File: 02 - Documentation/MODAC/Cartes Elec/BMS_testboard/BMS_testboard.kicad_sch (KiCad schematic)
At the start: 33 parts, among them J1 2P Droit 22-11-2022, J2 6P Droit 22-11-2062, J3 6P Droit 22-11-2062, J4 2P Droit 22-11-2022, Q1 NMOS SQ2348ES-T1_GE3, Q10 PMOS SI2343CDS-T1-GE3, Q11 NMOS SQ2348ES-T1_GE3, Q12 PMOS SI2343CDS-T1-GE3, Q13 NMOS SQ2348ES-T1_GE3, Q14 NMOS SQ2348ES-T1_GE3, Q15 PMOS SI2343CDS-T1-GE3, Q16 PMOS SI2343CDS-T1-GE3, Q17 NMOS SQ2348ES-T1_GE3, Q18 NMOS SQ2348ES-T1_GE3, Q19 PMOS SI2343CDS-T1-GE3, Q2 PMOS SI2343CDS-T1-GE3, Q20 PMOS SI2343CDS-T1-GE3, Q21 NMOS SQ2348ES-T1_GE3, Q22 NMOS SQ2348ES-T1_GE3, Q23 PMOS SI2343CDS-T1-GE3, Q24 PMOS SI2343CDS-T1-GE3, Q3 NMOS SQ2348ES-T1_GE3, Q4 PMOS SI2343CDS-T1-GE3, Q5 NMOS SQ2348ES-T1_GE3, Q6 PMOS SI2343CDS-T1-GE3, Q7 NMOS SQ2348ES-T1_GE3, Q8 PMOS SI2343CDS-T1-GE3, Q9 NMOS SQ2348ES-T1_GE3, U1 ADG406BPZ

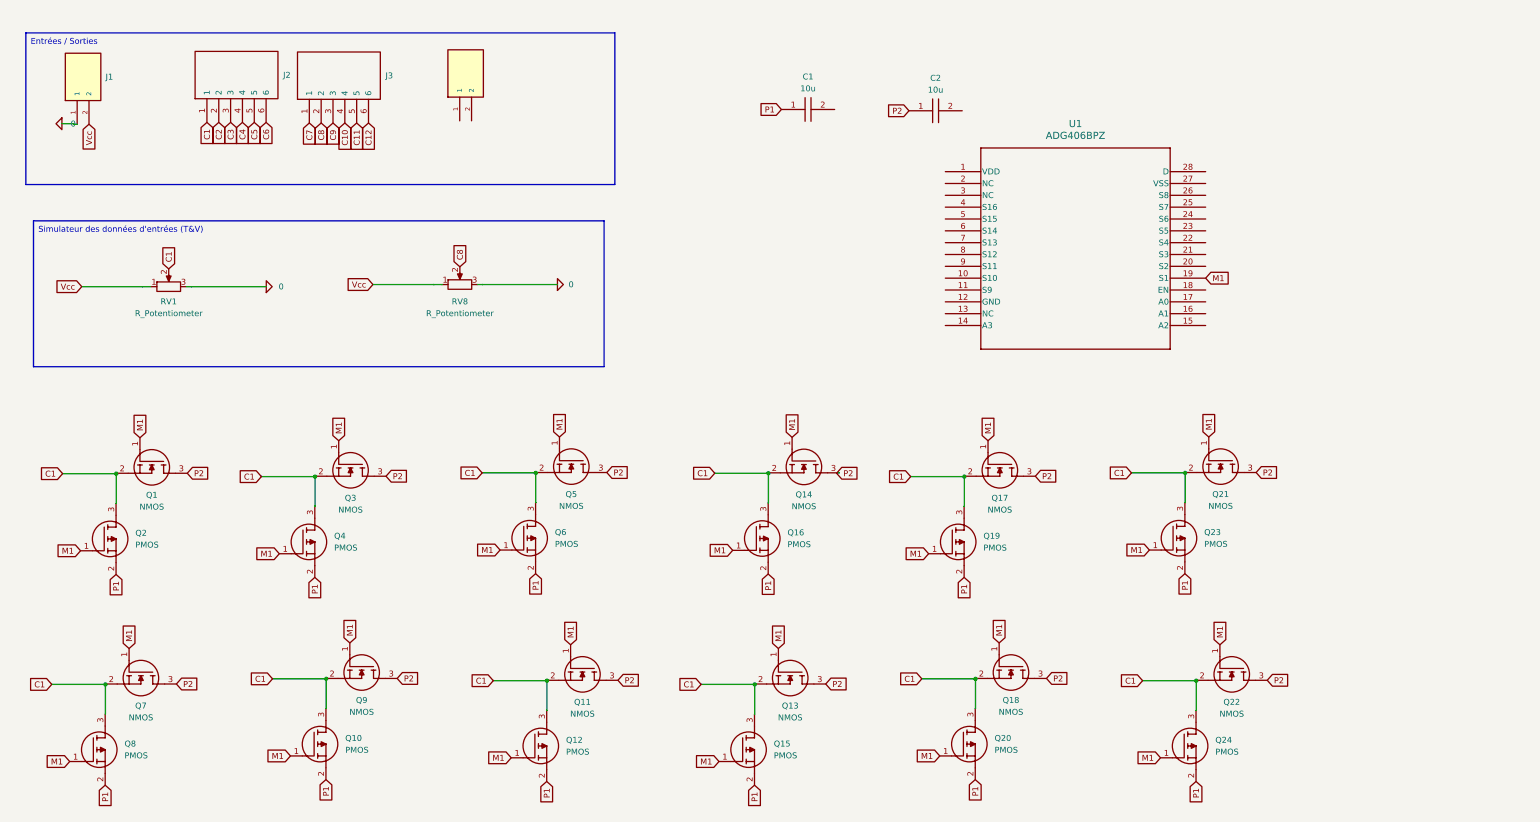
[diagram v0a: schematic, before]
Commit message: BOMs et BMS Testboard
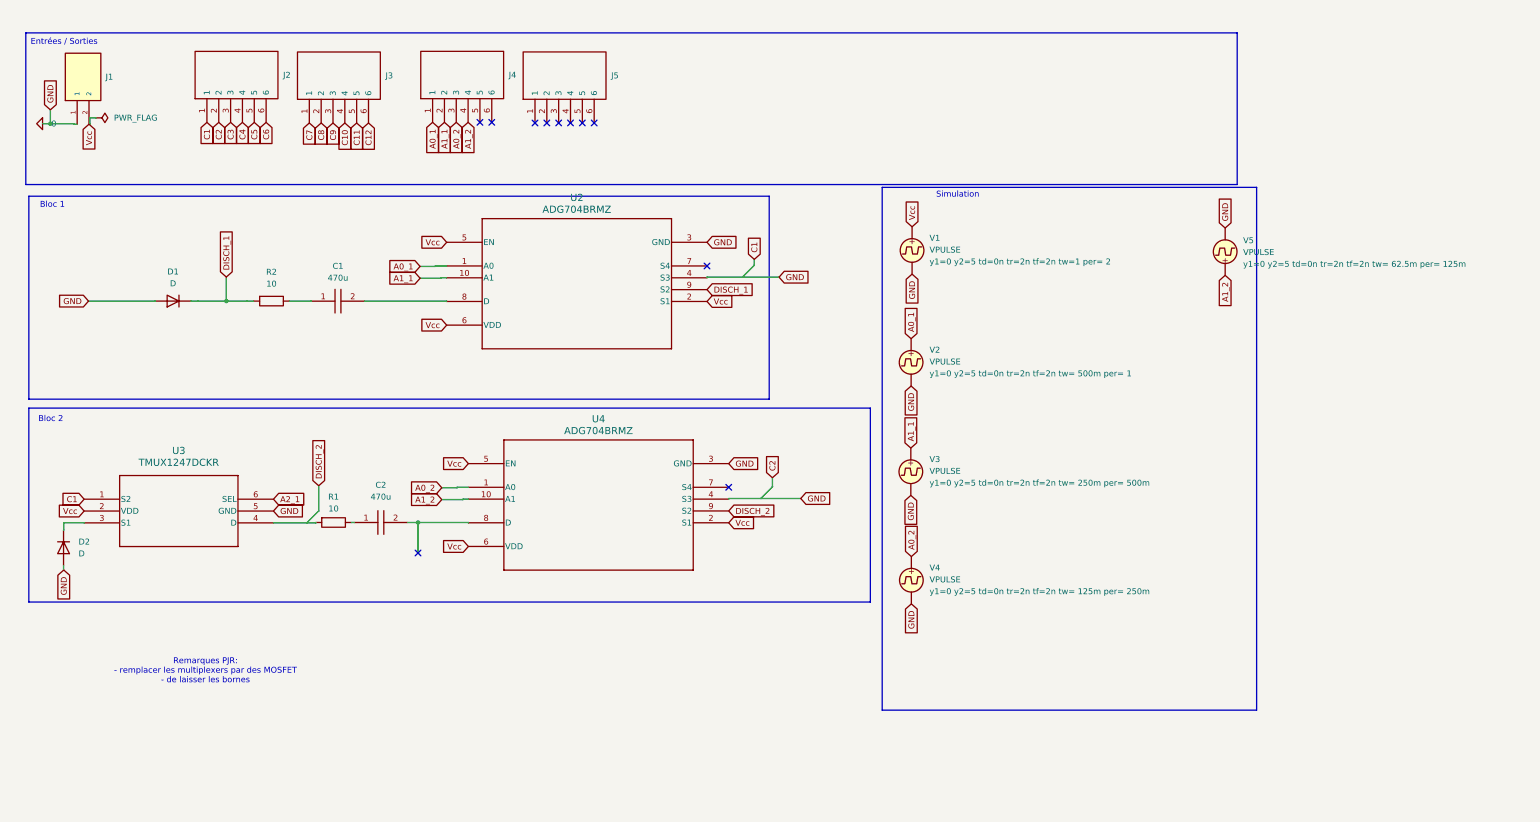
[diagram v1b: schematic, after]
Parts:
- removed J4: 2P Droit 22-11-2022, EPSA_lib:MOLEX_22-11-2022, symbol EPSA_lib:2P Droit 22-11-2022
- removed Q1, Q11, Q13, Q14, Q17, Q18, Q21, Q22, Q3, Q5, Q7, Q9: NMOS SQ2348ES-T1_GE3, EPSA_lib:SOT95P237X112-3N, symbol EPSA_lib:NMOS SQ2348ES-T1_GE3
- removed Q10, Q12, Q15, Q16, Q19, Q2, Q20, Q23, Q24, Q4, Q6, Q8: PMOS SI2343CDS-T1-GE3, EPSA_lib:SOT95P237X112-3N, symbol EPSA_lib:PMOS SI2343CDS-T1-GE3
- removed RV1, RV8: R_Potentiometer, symbol Device:R_Potentiometer
- removed U1: ADG406BPZ, P_28_ADI, symbol Multiplexer_16channels:ADG406BPZ
- added D1, D2: D, symbol Device:D
- added J4, J5: 6P Droit 22-11-2062, EPSA_lib:HDRV6W87P0X254_1X6_1509X635X1092P, symbol EPSA_lib:6P Droit 22-11-2062
- added R1, R2: 10, symbol Device:R
- added U2, U4: ADG704BRMZ, RM_10_ADI, symbol 2025-02-14_19-46-42:ADG704BRMZ
- added U3: TMUX1247DCKR, SOT-SC70_DCK_6_TEX, symbol 2025-02-14_19-49-50:TMUX1247DCKR
- added V1, V2, V3, V4, V5: VPULSE, symbol Simulation_SPICE:VPULSE
- C1, C2: value 10u -> 470u
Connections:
- net 0: now also D1.2 (A), D2.2 (A), U2.3 (GND), U2.4 (S3), U3.5 (GND), U4.3 (GND), U4.4 (S3), V1.2, V2.2, V3.2, V4.2, V5.2
- net C1: now also U3.1 (S2)
- net Vcc: now also U2.2 (S1), U2.5 (EN), U2.6 (VDD), U3.2 (VDD), U4.2 (S1), U4.5 (EN), U4.6 (VDD), V1.1
- net at C2.2: now also U4.8 (D)
- net at C1.2: now also U2.8 (D)
- net P1: no longer names the net of C1.1
- net P1: now also R2.1
- net P2: no longer names the net of C2.1
- net P2: now also R1.1
- new net: R1.2, U3.4 (D)
- new net: D2.1 (K), U3.3 (S1)
- new net A0_1: J4.1, U2.1 (A0), V2.1
- new net A0_2: J4.3, U4.1 (A0), V4.1
- new net A1_1: J4.2, U2.10 (A1), V3.1
- new net A1_2: J4.4, U4.10 (A1), V5.1
- new net A2_1: U3.6 (SEL)
- new net DISCH_1: D1.1 (K), R2.2, U2.9 (S2)
- new net DISCH_2: U4.9 (S2)
- no-connect marks 0 -> 11
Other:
- note added: "Bloc 1"
- note added: "Bloc 2"
- note added: "Remarques PJR: - remplacer les multiplexers par des MOSFET - de laisser les bornes"
- note added: "Simulation"

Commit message: BMS Testboard schematic finito
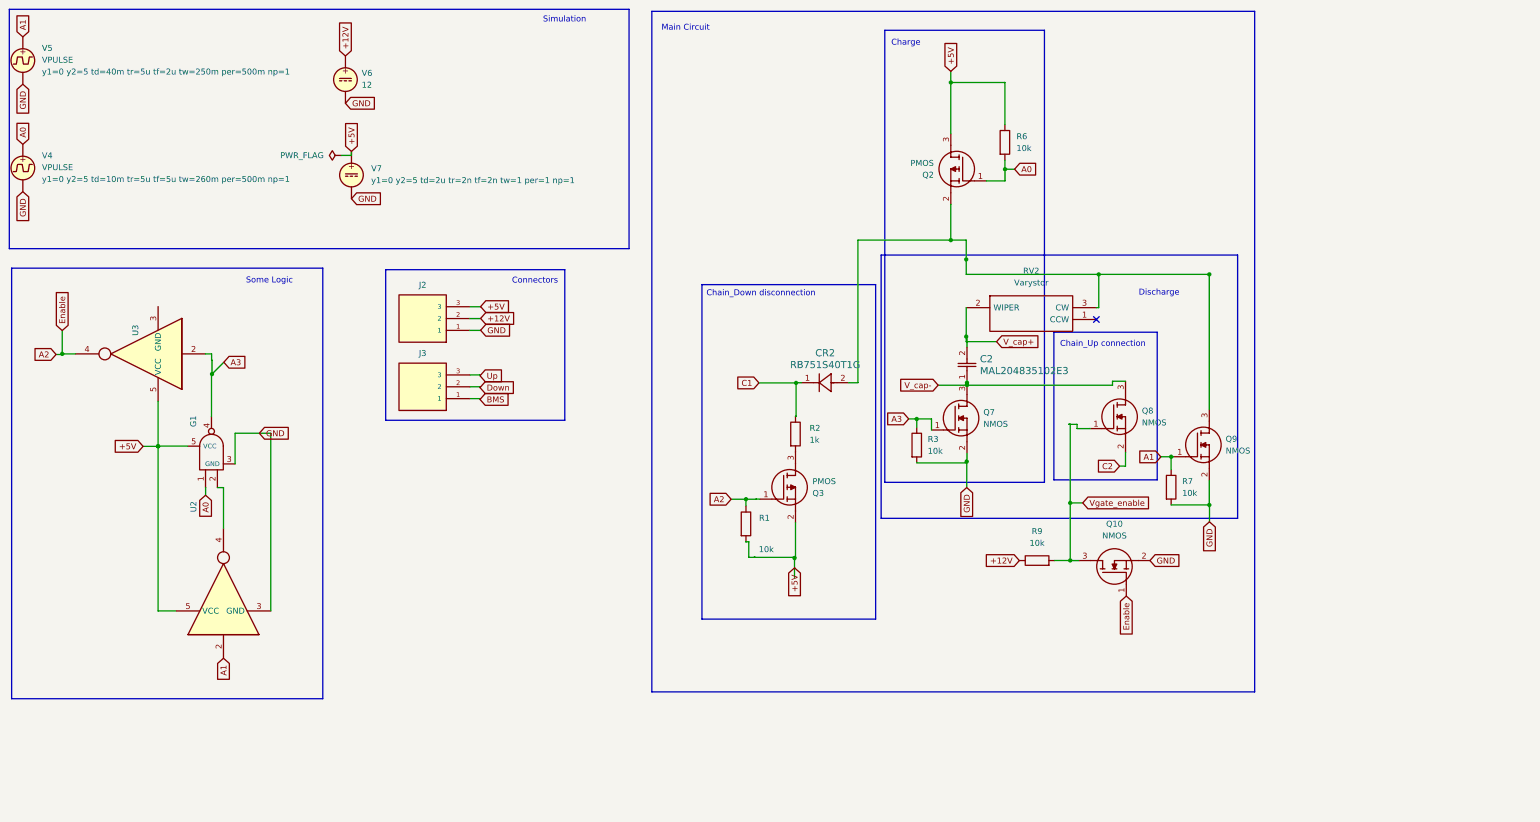
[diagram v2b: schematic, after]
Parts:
- removed C1, C2: 470u, EPSA_lib:CAPC2012X130N, symbol EPSA_lib:Condensateur 0805Y1000104JXT
- removed D1, D2: D, symbol Device:D
- removed J1: 2P Droit 22-11-2022, EPSA_lib:MOLEX_22-11-2022, symbol EPSA_lib:2P Droit 22-11-2022
- removed J2, J3, J4, J5: 6P Droit 22-11-2062, EPSA_lib:HDRV6W87P0X254_1X6_1509X635X1092P, symbol EPSA_lib:6P Droit 22-11-2062
- removed U2, U4: ADG704BRMZ, RM_10_ADI, symbol 2025-02-14_19-46-42:ADG704BRMZ
- removed U3: TMUX1247DCKR, SOT-SC70_DCK_6_TEX, symbol 2025-02-14_19-49-50:TMUX1247DCKR
- removed V1, V2, V3: VPULSE, symbol Simulation_SPICE:VPULSE
- added C2: MAL204835102E3, CAP_038RSU_10X20X.6_VIS, symbol 594-MAL204835102E3:MAL204835102E3
- added CR2: RB751S40T1G, DIODE_SOD523_1P3XP9_ONS, symbol RB751S40T1G:RB751S40T1G
- added G1: Gate NAND SN74AHCT1G00DBVR, EPSA_lib:SOT95P280X145-5N, symbol EPSA_Lib:Gate NAND SN74AHCT1G00DBVR
- added J2, J3: 3P Droit 22-11-2032, EPSA_lib:MOLEX_22-11-2032, symbol EPSA_Lib:3P Droit 22-11-2032
- added Q10, Q7, Q8, Q9: NMOS SQ2348ES-T1_GE3, EPSA_lib:SOT95P237X112-3N, symbol EPSA_Lib:NMOS SQ2348ES-T1_GE3
- added Q2, Q3: PMOS SI2343CDS-T1-GE3, EPSA_lib:SOT95P237X112-3N, symbol EPSA_Lib:PMOS SI2343CDS-T1-GE3
- added R3, R6, R7, R9: 10k, Resistor_SMD:R_1206_3216Metric_Pad1.30x1.75mm_HandSolder, symbol Device:R
- added RV2: Varystor 3296Y-1-223LF, EPSA_lib:3296Y1223LF, symbol EPSA_Lib:Varystor 3296Y-1-223LF
- added U2, U3: 74LVC1GU04DRL, Package_TO_SOT_SMD:SOT-553, symbol 74xGxx:74LVC1GU04DRL
- added V6: 12, symbol Simulation_SPICE:VDC
- added V7: ${SIM.PARAMS}, symbol Simulation_SPICE:VDC
- R1: value 10 -> 10k; footprint (none) -> Resistor_SMD:R_1206_3216Metric_Pad1.30x1.75mm_HandSolder
- R2: value 10 -> 1k; footprint (none) -> Resistor_SMD:R_1206_3216Metric_Pad1.30x1.75mm_HandSolder
- V4, V5: now left out of the parts list
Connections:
- net C1: now also R2.1, CR2.1
- net C2: now also Q8.2
- net A2: now reaches R1.1
- net A2: now also Q10.1, Q3.1, U3.4
- net +5V: now reaches R1.2
- net +5V: now also G1.5 (VCC), J2.3, Q2.3, Q3.2, R6.1, U2.5 (VCC), U3.5 (VCC), V7.1
- net 0 renamed GND
- net GND: now also G1.3 (GND), J2.1, Q10.2, Q7.2, Q9.2, R3.2, R7.2, U2.3 (GND), V6.2, V7.2
- net A0_2 renamed A0
- net A0: now also G1.1, Q2.1, R6.2
- net A1_2 renamed A1
- net A1: now also Q9.1, R7.1, U2.2
- net DISCH_1: no longer names the net of R2.2
- net DISCH_1: now also Q3.3
- new net: CR2.2, Q2.2, Q9.3, RV2.3 (CW)
- new net: G1.2, U2.4
- new net: G1.4, U3.2
- new net +12V: J2.2, R9.1, V6.1
- new net A3: Q7.1, R3.1
- new net BMS: J3.1
- new net Down: J3.2
- new net Up: J3.3
- new net V_cap+: C2.2, RV2.2 (WIPER)
- new net V_cap-: C2.1, Q7.3, Q8.3
- new net Vgate_enable: Q10.3, Q8.1, R9.2
- no-connect marks 11 -> 1
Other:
- note added: "Chain_Up connection"
- note added: "Charge"
- note added: "Connectors"
- note added: "Discharge"
- note added: "Main Circuit"
- note added: "Some Logic"
- note removed: "Bloc 1"
- note removed: "Bloc 2"
- note removed: "Remarques PJR: - remplacer les multiplexers par des MOSFET - de laisser les bornes"
